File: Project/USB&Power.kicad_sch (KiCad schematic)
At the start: 12 parts, among them J1 JST SH, J12 USB_C sink board 1.3mm, J2 Pico EZmate, U58 PRTR5V0U2X

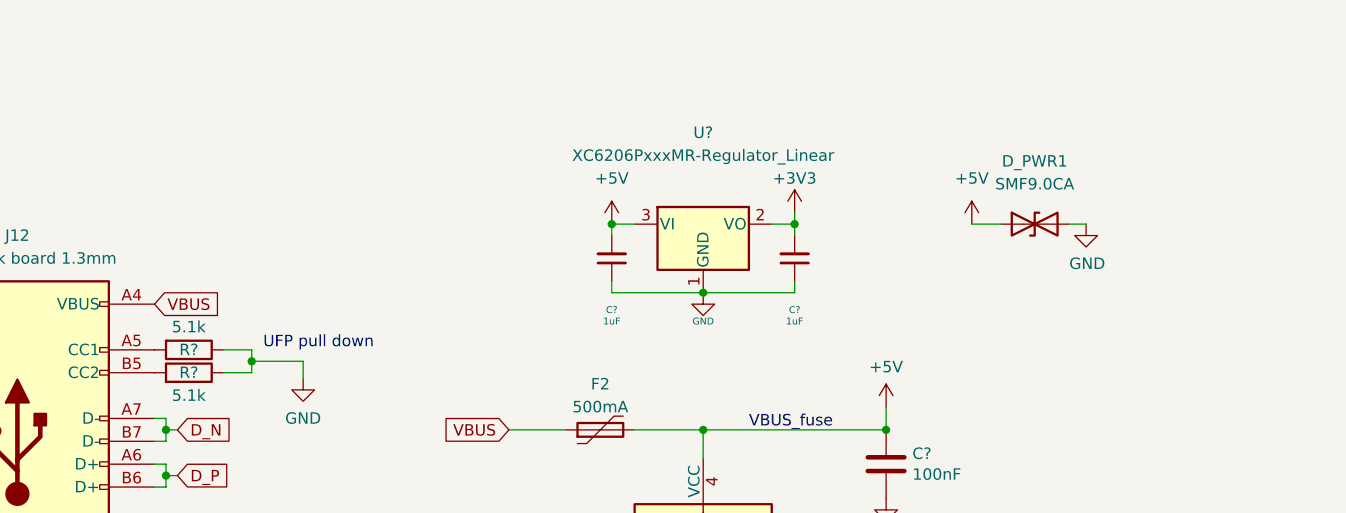
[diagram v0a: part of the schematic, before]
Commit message: revision work
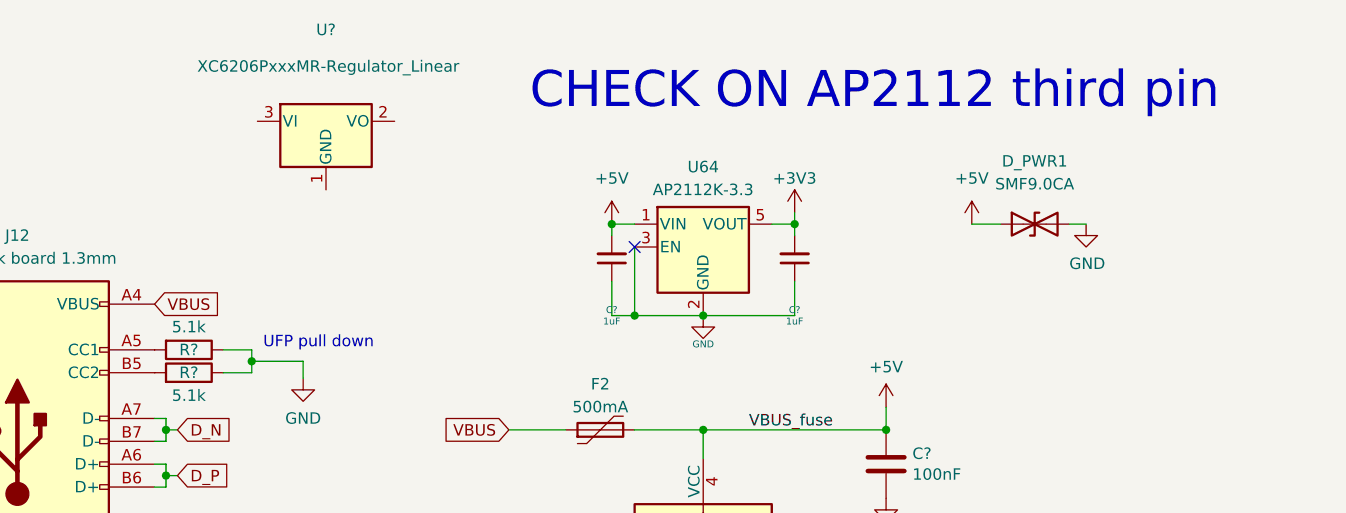
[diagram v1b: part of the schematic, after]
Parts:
- added U64: AP2112K-3.3, Package_TO_SOT_SMD:SOT-23-5, symbol Regulator_Linear:AP2112K-3.3
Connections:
- net +3V3: now also U64.5 (VOUT); no longer U?.2 (VO)
- net +5V: now also U64.1 (VIN); no longer U?.3 (VI)
- net GND: now also U64.2 (GND), U64.3 (EN); no longer U?.1 (GND)
- no-connect marks 2 -> 3
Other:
- note added: "CHECK ON AP2112 third pin"
- moved on the sheet: U?
